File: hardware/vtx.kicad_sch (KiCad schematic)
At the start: 58 parts, among them J1 U.FL, Q27 BC857BM, Q28 AP1606, U19 RTC6705, U20 SE5004L, U21 LP5912-3.3, U22 LP5907-2.85, X4 8MHz 10pF

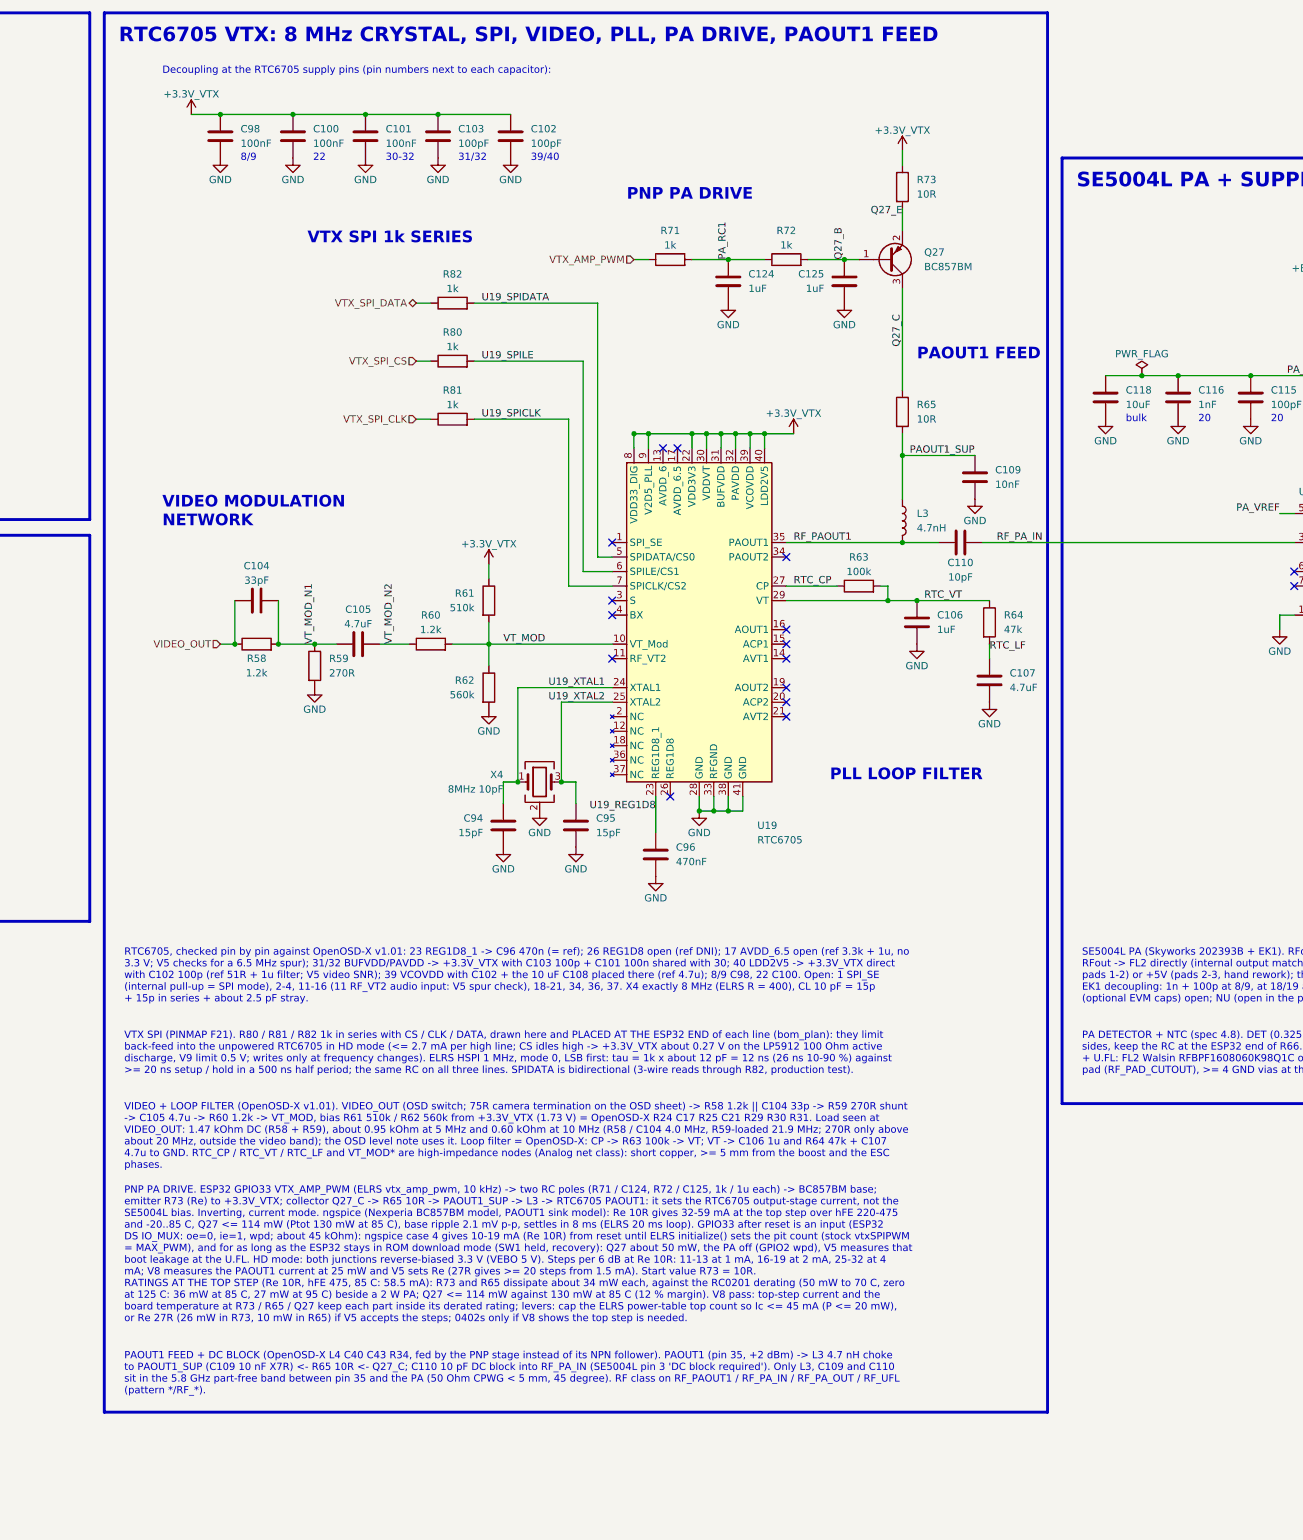
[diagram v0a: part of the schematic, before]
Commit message: WIP final schematic (D111/D113): further sheet and doc updates, PDF re-export; mid-run snapshot, not yet verified
Co-Authored-By: Claude Opus 5.5 <noreply@anthropic.com>
Claude-Session: https://claude.ai/code/session_01RFaS5jnC9tnPam9GBgmGnG
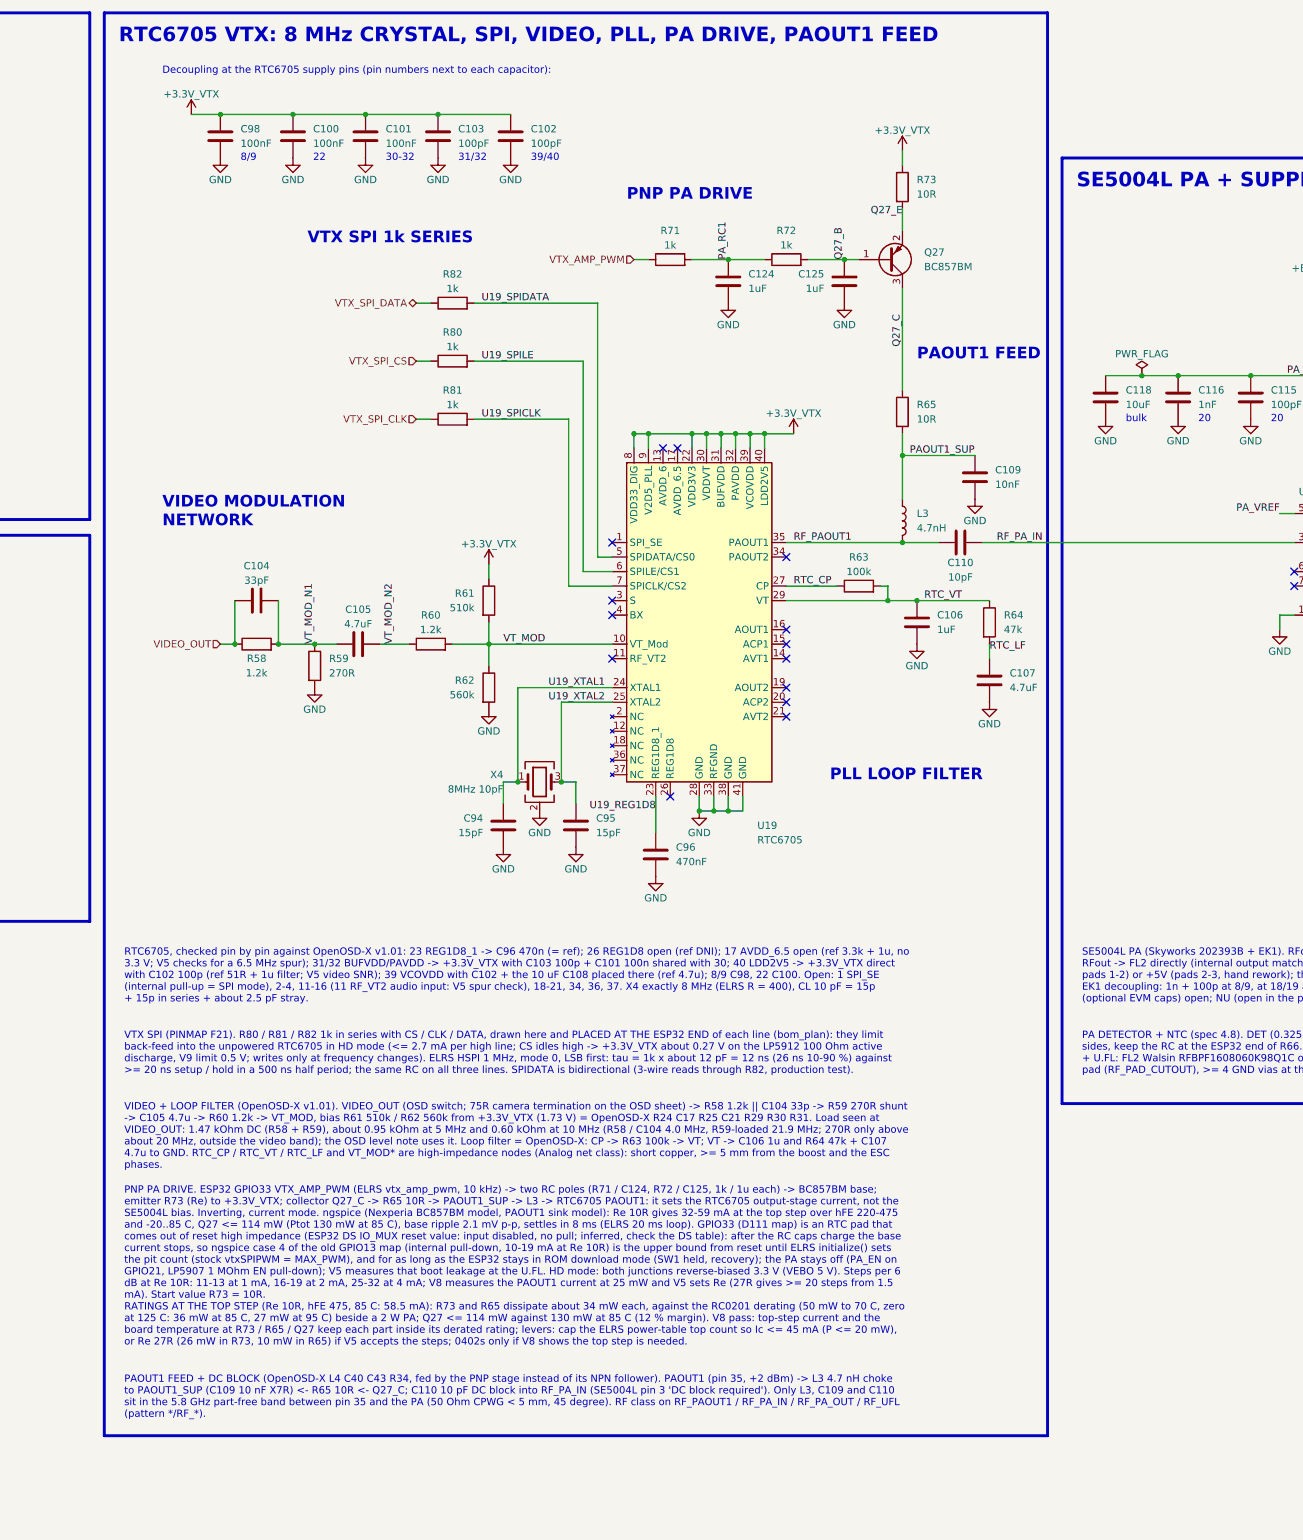
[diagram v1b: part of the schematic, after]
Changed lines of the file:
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@@
 	(rectangle
 		(start 137.16 27.94)
-		(end 302.26 272.86)
+		(end 302.26 276.98)
 		(stroke
 			(width 0.508)
@@
 		)
 	)
-	(text_box "PNP PA DRIVE. ESP32 GPIO33 VTX_AMP_PWM (ELRS vtx_amp_pwm, 10 kHz) -> two RC poles (R71 / C124, R72 / C125, 1k / 1u each) -> BC857BM base; emitter R73 (Re) to +3.3V_VTX; collector Q27_C -> R65 10R -> PAOUT1_SUP -> L3 -> RTC6705 PAOUT1: it sets the RTC6705 output-stage current, not the SE5004L bias. Inverting, current mode. ngspice (Nexperia BC857BM model, PAOUT1 sink model): Re 10R gives 32-59 mA at the top step over hFE 220-475 and -20..85 C, Q27 <= 114 mW (Ptot 130 mW at 85 C), base ripple 2.1 mV p-p, settles in 8 ms (ELRS 20 ms loop). GPIO33 after reset is an input (ESP32 DS IO_MUX: oe=0, ie=1, wpd; about 45 kOhm): ngspice case 4 gives 10-19 mA (Re 10R) from reset until ELRS initialize() sets the pit count (stock vtxSPIPWM = MAX_PWM), and for as long as the ESP32 stays in ROM download mode (SW1 held, recovery): Q27 about 50 mW, the PA off (GPIO2 wpd), V5 measures that boot leakage at the U.FL. HD mode: both junctions reverse-biased 3.3 V (VEBO 5 V). Steps per 6 dB at Re 10R: 11-13 at 1 mA, 16-19 at 2 mA, 25-32 at 4 mA; V8 measures the PAOUT1 current at 25 mW and V5 sets Re (27R gives >= 20 steps from 1.5 mA). Start value R73 = 10R.\nRATINGS AT THE TOP STEP (Re 10R, hFE 475, 85 C: 58.5 mA): R73 and R65 dissipate about 34 mW each, against the RC0201 derating (50 mW to 70 C, zero at 125 C: 36 mW at 85 C, 27 mW at 95 C) beside a 2 W PA; Q27 <= 114 mW against 130 mW at 85 C (12 % margin). V8 pass: top-step current and the board temperature at R73 / R65 / Q27 keep each part inside its derated rating; levers: cap the ELRS power-table top count so Ic <= 45 mA (P <= 20 mW), or Re 27R (26 mW in R73, 10 mW in R65) if V5 accepts the steps; 0402s only if V8 shows the top step is needed."
+	(text_box "PNP PA DRIVE. ESP32 GPIO33 VTX_AMP_PWM (ELRS vtx_amp_pwm, 10 kHz) -> two RC poles (R71 / C124, R72 / C125, 1k / 1u each) -> BC857BM base; emitter R73 (Re) to +3.3V_VTX; collector Q27_C -> R65 10R -> PAOUT1_SUP -> L3 -> RTC6705 PAOUT1: it sets the RTC6705 output-stage current, not the SE5004L bias. Inverting, current mode. ngspice (Nexperia BC857BM model, PAOUT1 sink model): Re 10R gives 32-59 mA at the top step over hFE 220-475 and -20..85 C, Q27 <= 114 mW (Ptot 130 mW at 85 C), base ripple 2.1 mV p-p, settles in 8 ms (ELRS 20 ms loop). GPIO33 (D111 map) is an RTC pad that comes out of reset high impedance (ESP32 DS IO_MUX reset value: input disabled, no pull; inferred, check the DS table): after the RC caps charge the base current stops, so ngspice case 4 of the old GPIO13 map (internal pull-down, 10-19 mA at Re 10R) is the upper bound from reset until ELRS initialize() sets the pit count (stock vtxSPIPWM = MAX_PWM), and for as long as the ESP32 stays in ROM download mode (SW1 held, recovery); the PA stays off (PA_EN on GPIO21, LP5907 1 MOhm EN pull-down); V5 measures that boot leakage at the U.FL. HD mode: both junctions reverse-biased 3.3 V (VEBO 5 V). Steps per 6 dB at Re 10R: 11-13 at 1 mA, 16-19 at 2 mA, 25-32 at 4 mA; V8 measures the PAOUT1 current at 25 mW and V5 sets Re (27R gives >= 20 steps from 1.5 mA). Start value R73 = 10R.\nRATINGS AT THE TOP STEP (Re 10R, hFE 475, 85 C: 58.5 mA): R73 and R65 dissipate about 34 mW each, against the RC0201 derating (50 mW to 70 C, zero at 125 C: 36 mW at 85 C, 27 mW at 95 C) beside a 2 W PA; Q27 <= 114 mW against 130 mW at 85 C (12 % margin). V8 pass: top-step current and the board temperature at R73 / R65 / Q27 keep each part inside its derated rating; levers: cap the ELRS power-table top count so Ic <= 45 mA (P <= 20 mW), or Re 27R (26 mW in R73, 10 mW in R65) if V5 accepts the steps; 0402s only if V8 shows the top step is needed."
 		(exclude_from_sim no)
 		(at 139.7 232.15 0)
-		(size 160.02 27.72)
+		(size 160.02 31.84)
 		(margins 0.9525 0.9525 0.9525 0.9525)
 		(stroke
@@
 	(text_box "PAOUT1 FEED + DC BLOCK (OpenOSD-X L4 C40 C43 R34, fed by the PNP stage instead of its NPN follower). PAOUT1 (pin 35, +2 dBm) -> L3 4.7 nH choke to PAOUT1_SUP (C109 10 nF X7R) <- R65 10R <- Q27_C; C110 10 pF DC block into RF_PA_IN (SE5004L pin 3 'DC block required'). Only L3, C109 and C110 sit in the 5.8 GHz part-free band between pin 35 and the PA (50 Ohm CPWG < 5 mm, 45 degree). RF class on RF_PAOUT1 / RF_PA_IN / RF_PA_OUT / RF_UFL (pattern */RF_*)."
 		(exclude_from_sim no)
-		(at 139.7 261.14 0)
+		(at 139.7 265.26 0)
 		(size 160.02 9.18)
 		(margins 0.9525 0.9525 0.9525 0.9525)
